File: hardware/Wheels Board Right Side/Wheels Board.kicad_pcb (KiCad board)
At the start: 2 copper layers, 92.9 x 69.7 mm, 46 parts, among them J1 Conn_01x05, J10 gnd, J11 hall_out, J12 Conn_01x05, J2 24v, J3 Conn_01x03, J4 53307-2471, J6 Conn_01x05_Pin, J7 Conn_01x07, J8 24v, J9 5v, U1 ASM330LHHTR, U2 XIAO-ESP32-S3-SMD, U4 TPS5405DR, U5 TLV9002QDRQ1

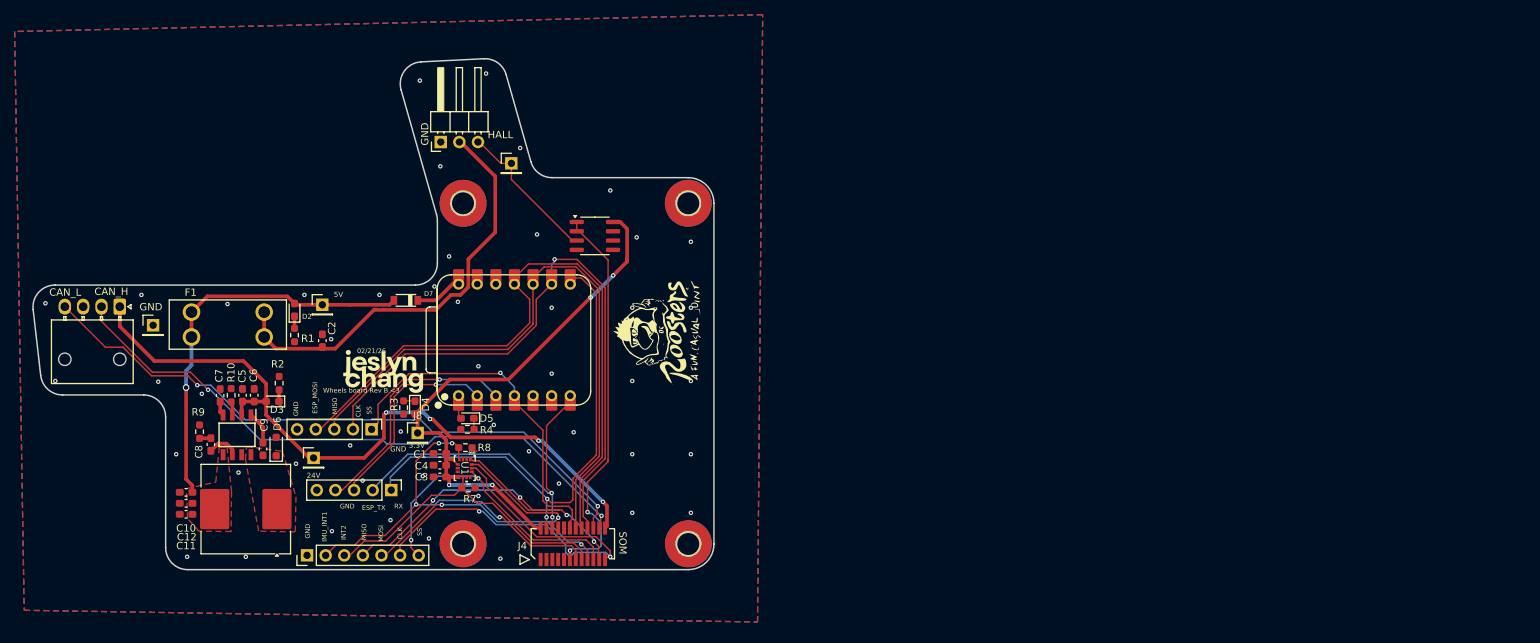
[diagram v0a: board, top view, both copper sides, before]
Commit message: added right side
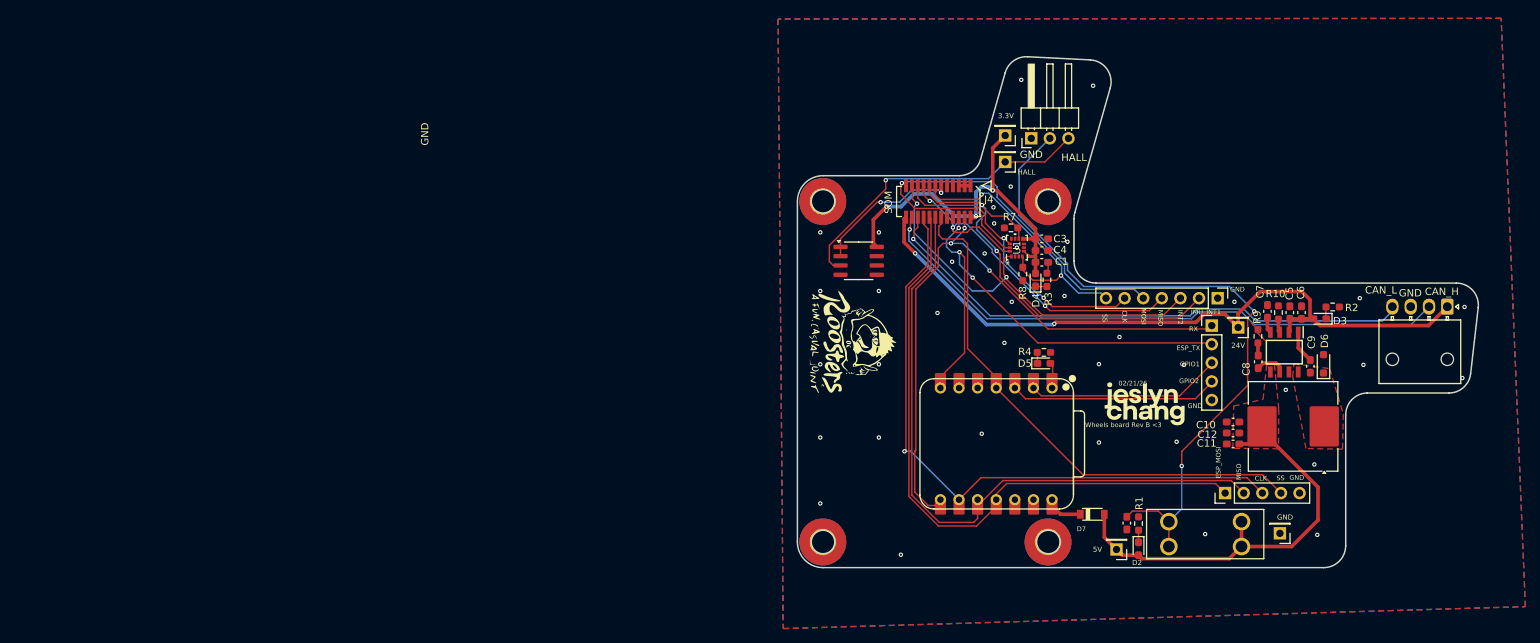
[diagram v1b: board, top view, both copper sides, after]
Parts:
- removed LOGO1: LHRS, UTSVT_Logos:LHRs_LOGO
- moved J6 181.2 mm to (246.2, 69.9)
- moved J10 156.4 mm to (223.4, 100.8), turned to 180 degrees
- moved R9 145.0 mm to (220.4, 73.9)
- moved R2 144.2 mm to (230.6, 69.9), turned to 0 degrees
- moved C7 143.4 mm to (221.7, 70.5)
- moved D6 143.4 mm to (229.4, 77.7)
- moved C9 143.4 mm to (227.6, 78.0)
- moved C5 143.4 mm to (224.8, 70.7)
- moved C6 143.4 mm to (226.4, 70.7)
- moved C8 143.4 mm to (220.4, 77.4)
- moved D3 143.4 mm to (228.9, 71.5)
- moved L1 143.4 mm to (225.2, 86.2)
- moved U4 143.4 mm to (224.0, 76.1)
- moved R10 143.4 mm to (223.2, 70.7)
- moved C10 143.2 mm to (217.0, 85.6)
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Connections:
- J1 pad 1: /ESP_SPI_SS -> /ESP_SPI_MOSI
- J1 pad 2: /ESP_SPI_CLK -> /ESP_SPI_MISO
- J1 pad 3: /ESP_SPI_MISO -> /ESP_SPI_CLK
- J1 pad 4: /ESP_SPI_MOSI -> /ESP_SPI_SS
- J7 pad 2: /IMU_INT1 -> /IMU_INT2
- J7 pad 3: /IMU_INT2 -> /IMU_SPI_MISO
- J7 pad 4: /IMU_SPI_MISO -> /IMU_SPI_MOSI
- J7 pad 5: /IMU_SPI_MOSI -> /IMU_SPI_CLK
- J7 pad 6: /IMU_SPI_CLK -> /IMU_SPI_SS
- J7 pad 7: /IMU_SPI_SS -> /IMU_INT1
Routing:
- net Net-(J3-Pin_2): track 58.9 -> 93.9 mm, vias 0 -> 2
- net /HALL_PSOM: track 54.1 -> 20.0 mm
- net /ESP_SPI_SS: track 48.4 -> 72.4 mm, vias 1 -> 0
- net /HALL_OUT: track 20.4 -> 43.3 mm, vias 0 -> 1
- net +3.3V: track 76.2 -> 53.4 mm, vias 4 -> 3
- net /ESP_UART_TX: track 47.7 -> 67.0 mm, vias 2 -> 3
- net /ESP_UART_RX: track 68.5 -> 86.7 mm, vias 2 -> 3
- net /IMU_INT2: track 43.2 -> 59.9 mm, vias 0 -> 2
- net /IMU_INT1: track 56.0 -> 40.1 mm, vias 4 -> 2
- net /CAN_L: track 87.3 -> 75.1 mm, vias 2 -> 1
- net /IMU_SPI_MISO: track 60.8 -> 54.3 mm, vias 4 -> 2
- net /ESP_SPI_MISO: track 84.1 -> 90.2 mm
- net GND: track 0.39 -> 6.20 mm, vias 49 -> 38
- net /EXTRA_GPIO2: track 32.7 -> 28.8 mm, vias 1 -> 0
- net /CAN_H: track 83.9 -> 80.9 mm, vias 2 -> 1
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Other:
- outline, holes or cut-outs redrawn
- board text added: "GPIO1"
- board text added: "GPIO2"
